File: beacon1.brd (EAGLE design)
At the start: 113 x 112.7 mm, 108 parts, among them IC1 NCP1117ST50T3G, IC6 LP2985-33DBVR, IC7 LMV358IDGKR, SW1 EG1319, T1 FDN340P, U1 FGPMMOPA6H, U2 MIC5225-3.3, U4 MIC5225-3.3, U5 MB85RC256VPF-G-JNERE2, X1 JST 2PH, Y1 CSTCE16M0V53-R0 16MHZ, Y2 32.768kHz (535-9166-2-ND)

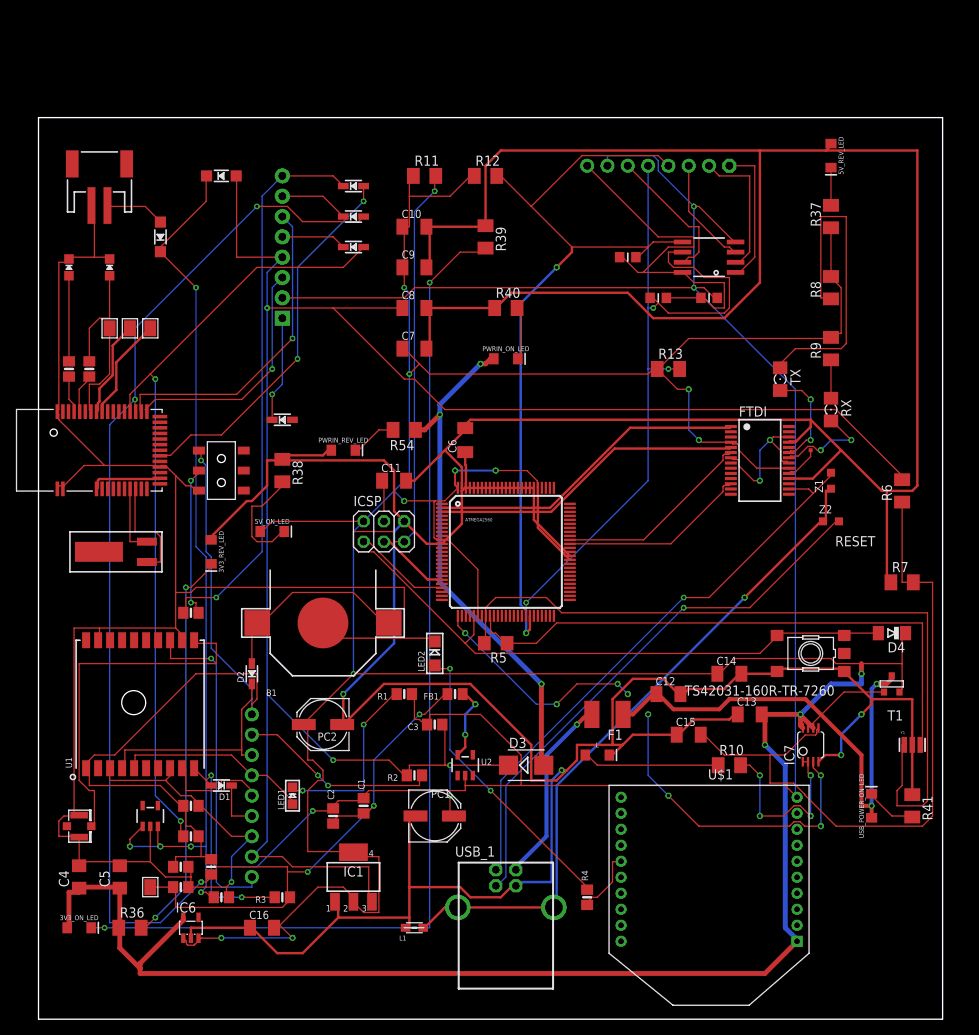
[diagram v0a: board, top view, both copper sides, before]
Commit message: save before leaving for meeting
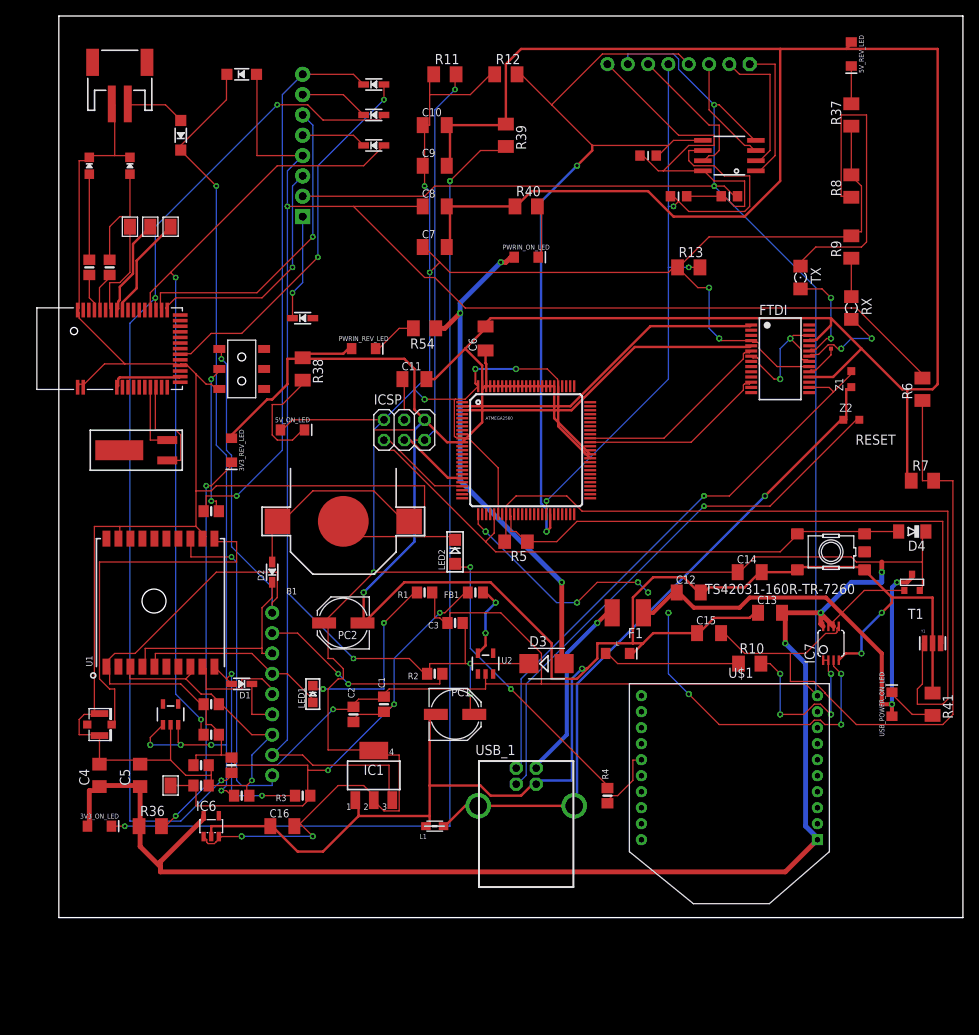
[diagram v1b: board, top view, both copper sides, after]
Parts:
- moved D11 13.0 mm to (30.5, 74.9)
- moved 3V3_REV_LED 13.0 mm to (21.6, 58.4)
- moved 5V_ON_LED 13.0 mm to (29.2, 61.0)
- moved 5V_REV_LED 13.0 mm to (99.1, 108.0)
- moved ATMEGA2560 13.0 mm to (58.4, 58.4)
- moved B1 13.0 mm to (35.6, 49.5)
- moved C10 13.0 mm to (47.0, 99.1)
- moved C11 13.0 mm to (44.5, 67.3)
- moved C13 13.0 mm to (88.9, 38.1)
- moved C15 13.0 mm to (81.3, 35.6)
- moved C6 13.0 mm to (53.3, 72.4)
- moved C8 13.0 mm to (47.0, 88.9)
- moved C9 13.0 mm to (47.0, 94.0)
- moved D10 13.0 mm to (39.4, 104.1)
- moved D12 13.0 mm to (22.9, 105.4)
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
